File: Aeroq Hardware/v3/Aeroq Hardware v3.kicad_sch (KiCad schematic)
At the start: 63 parts, among them Q1 Si1308EDL, U2 ESP32-C3-MINI-1-N4, U3 AMS1117-3.3, U4 SCD40-D-R1

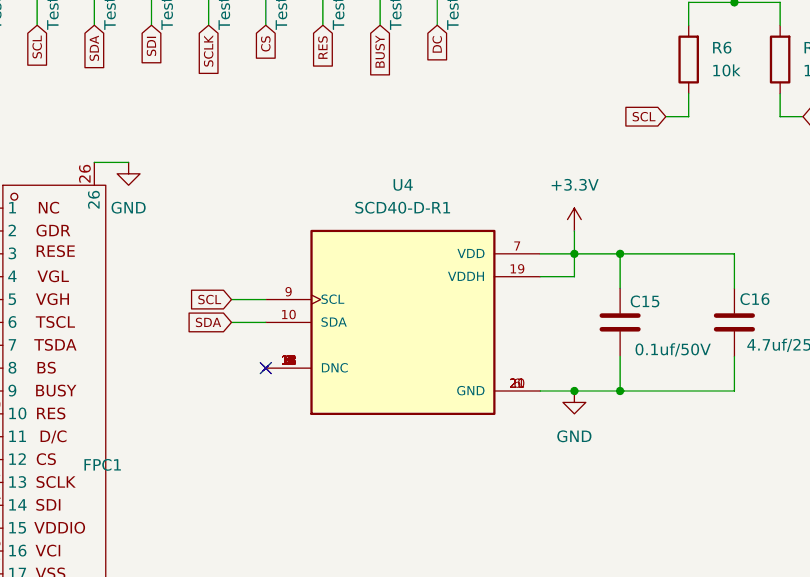
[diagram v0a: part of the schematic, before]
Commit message: PCB Updates
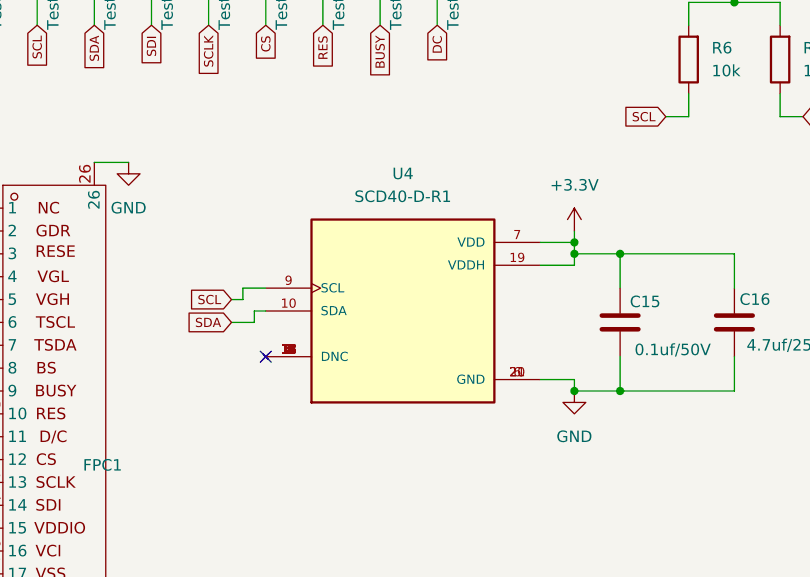
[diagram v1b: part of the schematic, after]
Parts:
- D2, D3, D4: footprint SOD-523_L1.2-W0.8-LS1.6-BI:SOD-523_L1.2-W0.8-LS1.6-BI -> Project Footprints:SOD-523_L1.2-W0.8-LS1.6-BI
- FPC1: footprint FPC-SMD_24P-P0.50_FPC-05FB-24PH20:FPC-SMD_24P-P0.50_FPC-05FB-24PH20 -> Project Footprints:FPC-SMD_24P-P0.50_FPC-05FB-24PH20
- SW1, SW2: footprint SW-SMD_L3.9-W3.0-P4.45:SW-SMD_L3.9-W3.0-P4.45 -> Project Footprints:SW-SMD_L3.9-W3.0-P4.45
- U1: footprint USBC_SMD_VERTICAL:TYPE-C-SMD_USB4120-03-C -> Project Footprints:TYPE-C-SMD_USB4120-03-C
- U2: footprint custom_footprints:XCVR_ESP32-C3-MINI-1-N4 -> Project Footprints:XCVR_ESP32-C3-MINI-1-N4
- U4: footprint Sensor:Sensirion_SCD4x-1EP_10.1x10.1mm_P1.25mm_EP4.8x4.8mm -> Project Footprints:XDCR_SCD40-D-R1
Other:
- moved on the sheet: U4
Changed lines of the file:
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@@
 	)
 	(junction
+		(at 213.36 134.62)
+		(diameter 0)
+		(color 0 0 0 0)
+	)
+	(junction
 		(at 38.1 67.31)
 		(diameter 0)
@@
 	)
 	(no_connect
-		(at 179.07 148.59)
+		(at 179.07 147.32)
 	)
 	(wire
@@
 	(wire
 		(pts
-			(xy 175.26 143.51) (xy 179.07 143.51)
+			(xy 177.8 142.24) (xy 179.07 142.24)
 		)
 		(stroke
@@
 	(wire
 		(pts
-			(xy 209.55 135.89) (xy 213.36 135.89)
+			(xy 209.55 134.62) (xy 213.36 134.62)
 		)
 		(stroke
@@
 	(wire
 		(pts
+			(xy 213.36 149.86) (xy 213.36 151.13)
+		)
+		(stroke
+			(width 0)
+			(type default)
+		)
+	)
+	(wire
+		(pts
 			(xy 34.29 39.37) (xy 34.29 15.24)
 		)
@@
 	(wire
 		(pts
-			(xy 213.36 138.43) (xy 209.55 138.43)
+			(xy 213.36 137.16) (xy 209.55 137.16)
 		)
 		(stroke
@@
 	(wire
 		(pts
-			(xy 175.26 140.97) (xy 179.07 140.97)
+			(xy 176.53 139.7) (xy 179.07 139.7)
 		)
 		(stroke
@@
 	(wire
 		(pts
-			(xy 209.55 151.13) (xy 213.36 151.13)
+			(xy 209.55 149.86) (xy 213.36 149.86)
 		)
 		(stroke
@@
 	(wire
 		(pts
+			(xy 177.8 142.24) (xy 177.8 143.51)
+		)
+		(stroke
+			(width 0)
+			(type default)
+		)
+	)
+	(wire
+		(pts
 			(xy 260.35 67.31) (xy 261.62 67.31)
 		)
@@
 	(wire
 		(pts
+			(xy 213.36 134.62) (xy 213.36 135.89)
+		)
+		(stroke
+			(width 0)
+			(type default)
+		)
+	)
+	(wire
+		(pts
 			(xy 231.14 107.95) (xy 231.14 106.68)
 		)
@@
 	(wire
 		(pts
+			(xy 176.53 139.7) (xy 176.53 140.97)
+		)
+		(stroke
+			(width 0)
+			(type default)
+		)
+	)
+	(wire
+		(pts
 			(xy 57.15 175.26) (xy 64.77 175.26)
 		)
@@
 	(wire
 		(pts
+			(xy 176.53 140.97) (xy 175.26 140.97)
+		)
+		(stroke
+			(width 0)
+			(type default)
+		)
+	)
+	(wire
+		(pts
 			(xy 109.22 176.53) (xy 130.81 176.53)
 		)
@@
 	(wire
 		(pts
-			(xy 213.36 133.35) (xy 213.36 135.89)
+			(xy 213.36 133.35) (xy 213.36 134.62)
 		)
 		(stroke
@@
 	(wire
 		(pts
-			(xy 213.36 135.89) (xy 213.36 138.43)
+			(xy 213.36 135.89) (xy 213.36 137.16)
 		)
 		(stroke
@@
 	(wire
 		(pts
+			(xy 177.8 143.51) (xy 175.26 143.51)
+		)
+		(stroke
+			(width 0)
+			(type default)
+		)
+	)
+	(wire
+		(pts
 			(xy 138.43 176.53) (xy 147.32 176.53)
 		)
@@
 			)
 		)
-		(property "Footprint" "SW-SMD_L3.9-W3.0-P4.45:SW-SMD_L3.9-W3.0-P4.45"
+		(property "Footprint" "Project Footprints:SW-SMD_L3.9-W3.0-P4.45"
 			(at 135.89 72.39 0)
 			(effects
@@
 			)
 		)
-		(property "Footprint" "SOD-523_L1.2-W0.8-LS1.6-BI:SOD-523_L1.2-W0.8-LS1.6-BI"
+		(property "Footprint" "Project Footprints:SOD-523_L1.2-W0.8-LS1.6-BI"
 			(at 90.17 59.69 0)
 			(effects
@@
 			)
 		)
-		(property "Footprint" "USBC_SMD_VERTICAL:TYPE-C-SMD_USB4120-03-C"
+		(property "Footprint" "Project Footprints:TYPE-C-SMD_USB4120-03-C"
 			(at 52.07 46.99 0)
 			(effects
@@
 			)
 		)
-		(property "Footprint" "SOD-523_L1.2-W0.8-LS1.6-BI:SOD-523_L1.2-W0.8-LS1.6-BI"
+		(property "Footprint" "Project Footprints:SOD-523_L1.2-W0.8-LS1.6-BI"
 			(at 82.55 59.69 0)
 			(effects
@@
 			)
 		)
-		(property "Footprint" "SOD-523_L1.2-W0.8-LS1.6-BI:SOD-523_L1.2-W0.8-LS1.6-BI"
+		(property "Footprint" "Project Footprints:SOD-523_L1.2-W0.8-LS1.6-BI"
 			(at 96.52 59.69 0)
 			(effects
@@
 			)
 		)
-		(property "Footprint" "SW-SMD_L3.9-W3.0-P4.45:SW-SMD_L3.9-W3.0-P4.45"
+		(property "Footprint" "Project Footprints:SW-SMD_L3.9-W3.0-P4.45"
 			(at 135.89 34.29 0)
 			(effects
@@
 			)
 		)
-		(property "Footprint" "custom_footprints:XCVR_ESP32-C3-MINI-1-N4"
+		(property "Footprint" "Project Footprints:XCVR_ESP32-C3-MINI-1-N4"
 			(at 242.57 64.77 0)
 			(effects
@@
 	(symbol
 		(lib_id "SCD40-D-R1:SCD40-D-R1")
-		(at 194.31 143.51 0)
+		(at 194.31 142.24 0)
 		(unit 1)
 		(exclude_from_sim no)
@@
 		(fields_autoplaced yes)
 		(property "Reference" "U4"
-			(at 194.31 128.27 0)
+			(at 194.31 127 0)
 			(effects
 				(font
@@
 		)
 		(property "Value" "SCD40-D-R1"
-			(at 194.31 130.81 0)
+			(at 194.31 129.54 0)
 			(effects
 				(font
@@
 			)
 		)
-		(property "Footprint" "Sensor:Sensirion_SCD4x-1EP_10.1x10.1mm_P1.25mm_EP4.8x4.8mm"
-			(at 194.31 143.51 0)
+		(property "Footprint" "Project Footprints:XDCR_SCD40-D-R1"
+			(at 194.31 142.24 0)
 			(effects
 				(font
@@
 		)
 		(property "Datasheet" ""
-			(at 194.31 143.51 0)
+			(at 194.31 142.24 0)
 			(effects
 				(font
@@
 		)
 		(property "Description" ""
-			(at 194.31 143.51 0)
+			(at 194.31 142.24 0)
 			(effects
 				(font
@@
 		)
 		(property "MF" "Sensirion AG"
-			(at 194.31 143.51 0)
+			(at 194.31 142.24 0)
 			(effects
 				(font
@@
 		)
 		(property "MAXIMUM_PACKAGE_HEIGHT" "6.8mm"
-			(at 194.31 143.51 0)
+			(at 194.31 142.24 0)
 			(effects
 				(font
@@
 		)
 		(property "Package" "None"
-			(at 194.31 143.51 0)
+			(at 194.31 142.24 0)
 			(effects
 				(font
@@
 		)
 		(property "Price" "None"
-			(at 194.31 143.51 0)
+			(at 194.31 142.24 0)
 			(effects
 				(font
@@
 		)
 		(property "Check_prices" "https://www.snapeda.com/parts/SCD40-D-R1/Sensirion/view-part/?ref=eda"
-			(at 194.31 143.51 0)
+			(at 194.31 142.24 0)
 			(effects
 				(font
@@
 		)
 		(property "STANDARD" "Manufacturer Recommendations"
-			(at 194.31 143.51 0)
+			(at 194.31 142.24 0)
 			(effects
 				(font
@@
 		)
 		(property "PARTREV" "1.2"
-			(at 194.31 143.51 0)
+			(at 194.31 142.24 0)
 			(effects
 				(font
@@
 		)
 		(property "SnapEDA_Link" "https://www.snapeda.com/parts/SCD40-D-R1/Sensirion/view-part/?ref=snap"
-			(at 194.31 143.51 0)
+			(at 194.31 142.24 0)
 			(effects
 				(font
@@
 		)
 		(property "MP" "SCD40-D-R1"
-			(at 194.31 143.51 0)
+			(at 194.31 142.24 0)
 			(effects
 				(font
@@
 		)
 		(property "Description_1" "Carbon Dioxide (CO2), Humidity, Temperature Sensor I2C"
-			(at 194.31 143.51 0)
+			(at 194.31 142.24 0)
 			(effects
 				(font
@@
 		)
 		(property "SNAPEDA_PN" "SCD41-D-R2"
-			(at 194.31 143.51 0)
+			(at 194.31 142.24 0)
 			(effects
 				(font
@@
 		)
 		(property "Availability" "In Stock"
-			(at 194.31 143.51 0)
+			(at 194.31 142.24 0)
 			(effects
 				(font
@@
 		)
 		(property "MANUFACTURER" "Sensirion"
-			(at 194.31 143.51 0)
+			(at 194.31 142.24 0)
 			(effects
 				(font
@@
 			)
 		)
-		(property "Footprint" "FPC-SMD_24P-P0.50_FPC-05FB-24PH20:FPC-SMD_24P-P0.50_FPC-05FB-24PH20"
+		(property "Footprint" "Project Footprints:FPC-SMD_24P-P0.50_FPC-05FB-24PH20"
 			(at 152.4 160.02 0)
 			(effects
